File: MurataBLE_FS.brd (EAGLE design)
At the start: 90 x 63 mm, 51 parts, among them CON2 C-2395.microSD, IC1 74LVC1G00DBV, IC2 IC_DCDC_LM27313, IC3 IC_LPC11U3XQFN33, IC4 IC_LDO_XX1117_4, IC5 1265-1139-1-ND, Q1 CLOCK_CRYSTAL_4_3225, SW1 SW_TACTSW_2PP8073, SW2 SW_TACTSW_2PP8073, SW3 SW_TACTSW_2PP8073, U1 IC_BLE_LBCA2HNZYZ-711, X1 TSW-102-02-S-S

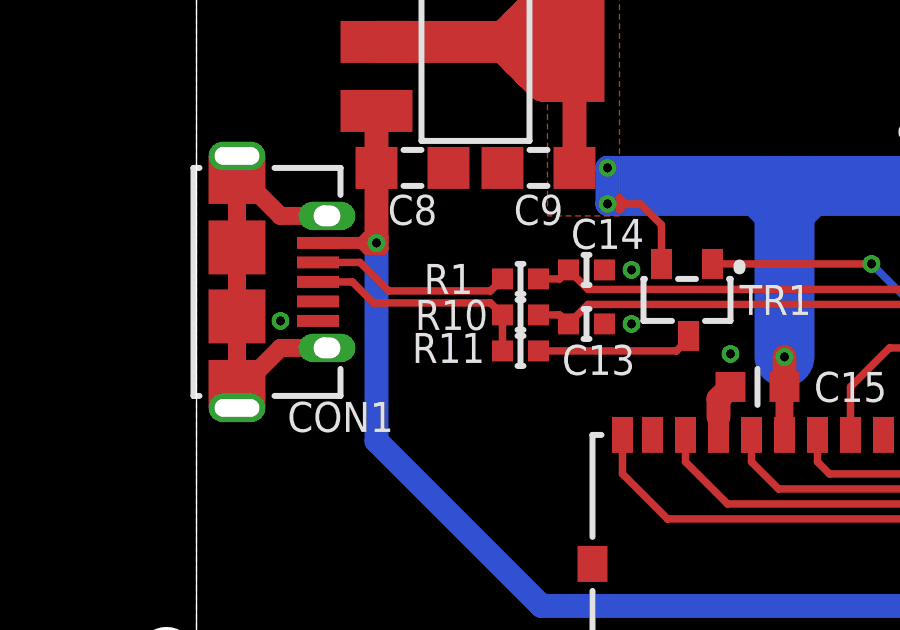
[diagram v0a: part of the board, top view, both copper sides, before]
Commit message: [ FS ] silk move
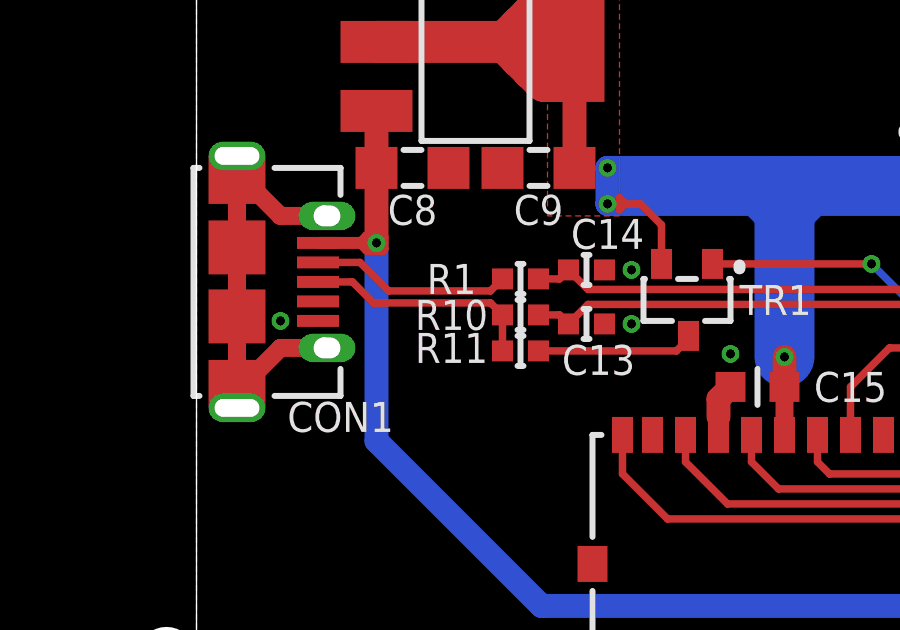
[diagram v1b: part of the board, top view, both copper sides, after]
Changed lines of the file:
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@@
 </element>
 <element name="R1" library="mylib" package="C0402" value="33/1005" x="20.8" y="31.6" smashed="yes">
-<attribute name="NAME" x="18.4" y="31.6" size="1" layer="25" font="vector" ratio="20" align="center"/>
+<attribute name="NAME" x="18.5" y="31.6" size="1" layer="25" font="vector" ratio="20" align="center"/>
 <attribute name="VALUE" x="20.2" y="29.7" size="1" layer="27" font="vector" ratio="20"/>
 </element>
@@
 </element>
 <element name="R11" library="mylib" package="C0402" value="1.5k/1005" x="20.8" y="29.2" smashed="yes" rot="R180">
-<attribute name="NAME" x="18.4" y="29.3" size="1" layer="25" font="vector" ratio="20" align="center"/>
+<attribute name="NAME" x="18.5" y="29.3" size="1" layer="25" font="vector" ratio="20" align="center"/>
 <attribute name="VALUE" x="21.4" y="31.1" size="1" layer="27" font="vector" ratio="20" rot="R180"/>
 </element>
